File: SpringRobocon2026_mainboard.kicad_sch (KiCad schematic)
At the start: 68 parts, among them J1 Conn_01x05_Socket_Encoder1, J10 Conn_01x04_Pin, J11 Conn_01x03_Pin, J12 Conn_01x03_Pin, J2 Conn_01x05_Socket_Encoder3, J3 Conn_01x05_Socket_Encoder5, J4 FDCAN_1, J5 Conn_01x05_Socket_Encoder2, J6 Conn_01x05_Socket_Encoder4, J7 FDCAN_2, J8 SOLENOID1, J9 Conn_01x02_Pin, Q1 MTA100N10KRI3, SW1 SW_DIP_x02_CANnum, U1 XT60_M, U2 ATA6561, U3 BA50BC0FP, U4 BA033CC0FP, U5 ATA6561, U6 NUCLEO-F446RE

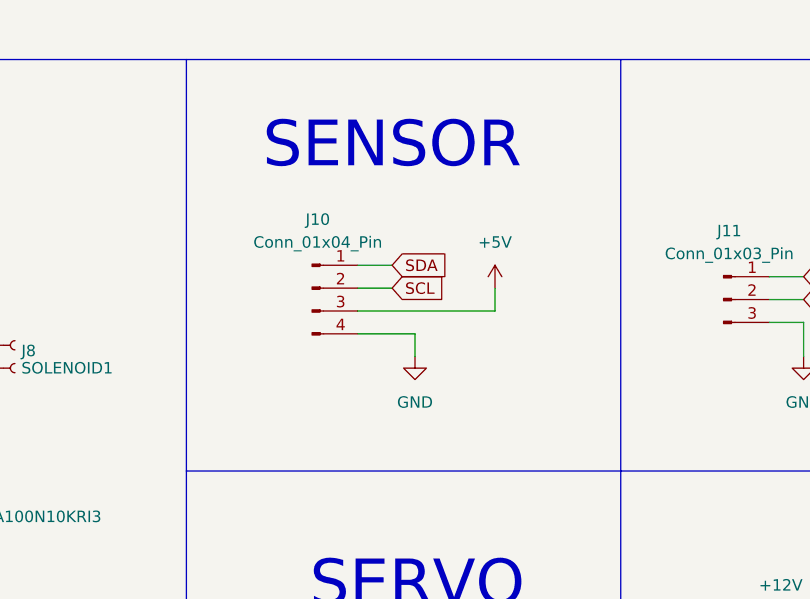
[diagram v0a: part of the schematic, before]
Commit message: 4回目修正
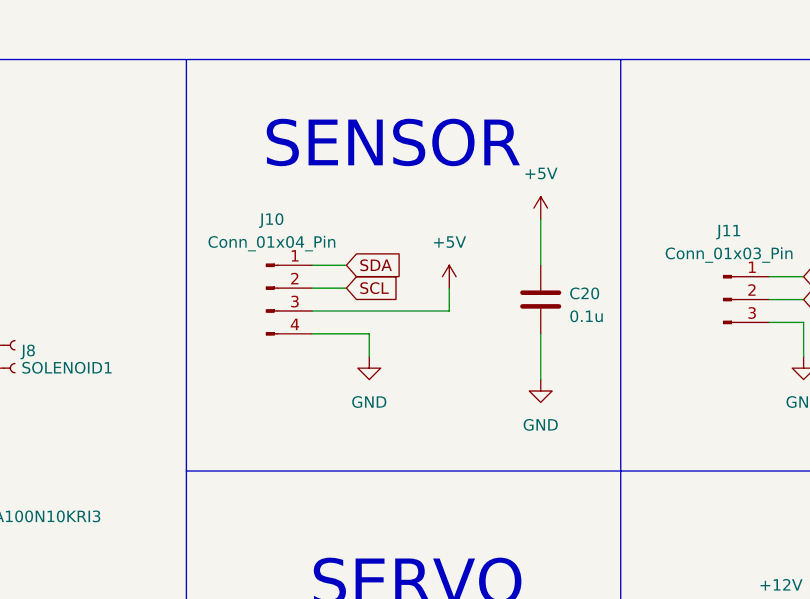
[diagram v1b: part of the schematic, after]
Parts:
- added C20: 0.1u, Capacitor_SMD:C_0603_1608Metric_Pad1.08x0.95mm_HandSolder, symbol Device:C
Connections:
- net +5V: now also C20.1
- net GND: now also C20.2
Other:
- moved on the sheet: J10
